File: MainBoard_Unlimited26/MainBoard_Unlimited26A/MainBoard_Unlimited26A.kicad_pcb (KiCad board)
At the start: 2 copper layers, 95 x 60 mm, 39 parts, among them J1 XT, J2 Screw_Terminal_01x02, J3 BAT, J4 EN, J5 UART, J6 UART, J7 VL5, P1 MP1584, P2 SERVO, Q1 IRFZ44N, U11 ACS712xLCTR-05B, U7 ESP32-DEVKIT-V1, U8 MPU6050/BNO085 I2C, U9 AMS1117-3.3

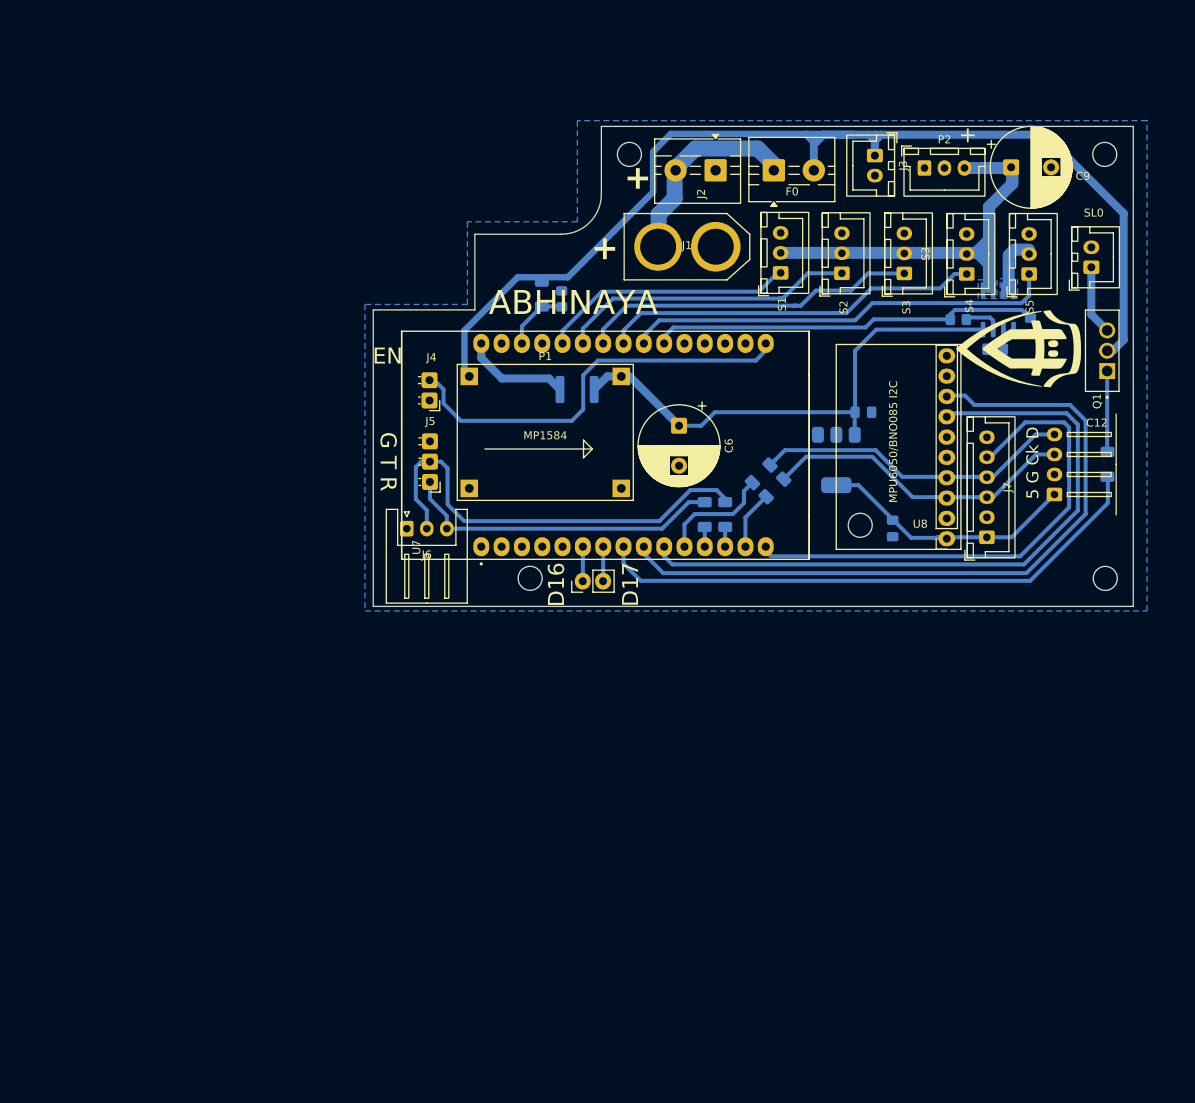
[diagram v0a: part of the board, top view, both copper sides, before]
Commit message: REV ALL
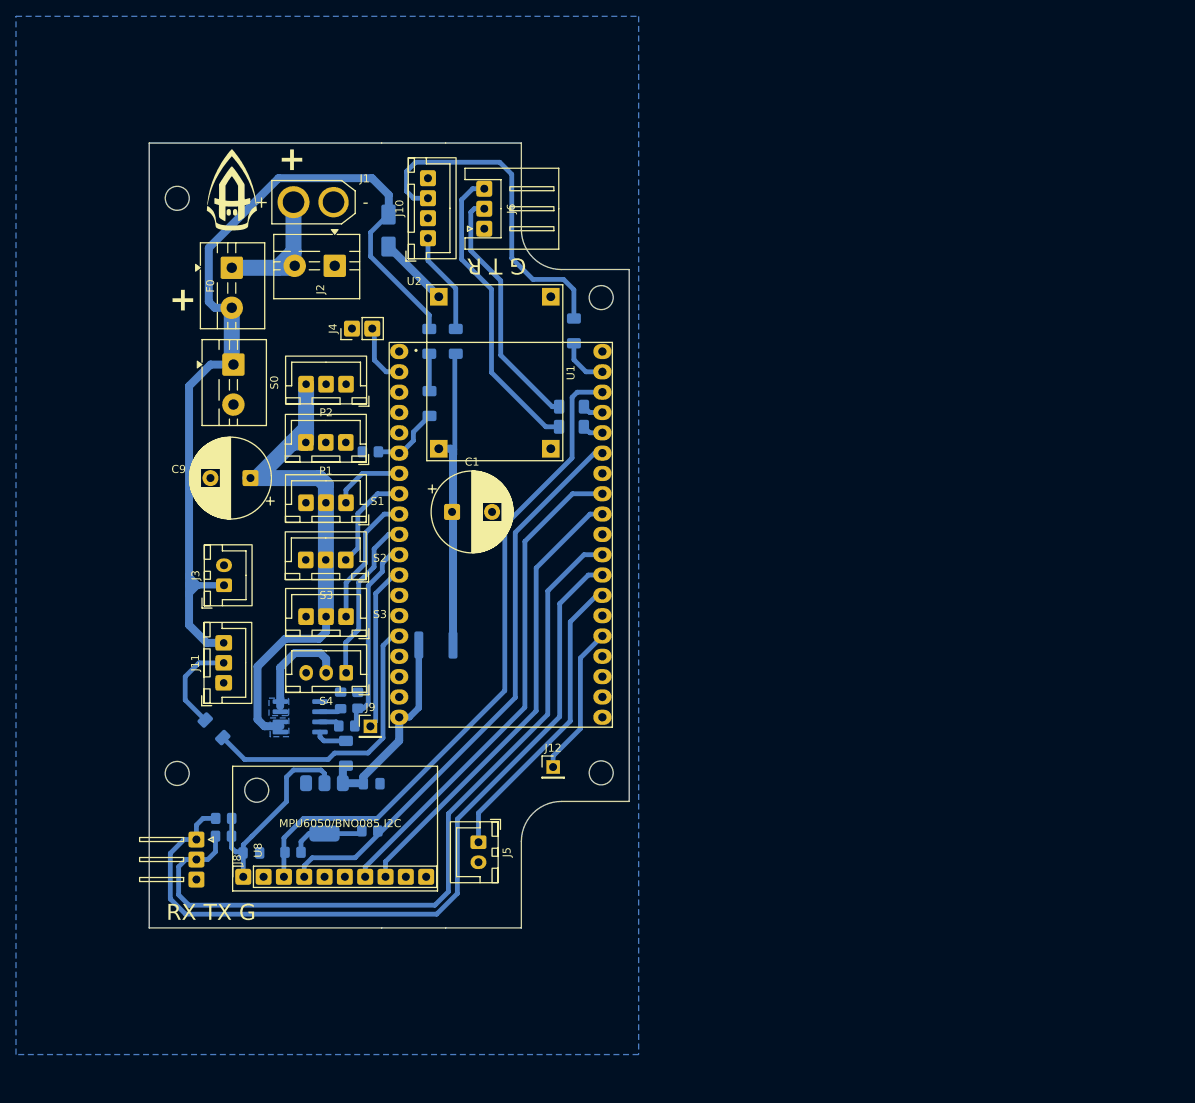
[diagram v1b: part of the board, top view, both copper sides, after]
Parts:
- removed C12: AB conn, Connector_JST:JST_XH_S4B-XH-A-1_1x04_P2.50mm_Horizontal
- removed C6: 1000uF, Capacitor_THT:CP_Radial_D10.0mm_P5.00mm
- removed D16: pin, Connector_PinHeader_2.54mm:PinHeader_1x02_P2.54mm_Vertical
- removed F6: Polyfuse, Fuse:Fuse_1812_4532Metric
- removed J7: VL5, Connector_JST:JST_XH_B6B-XH-A_1x06_P2.50mm_Vertical
- removed Q1: IRFZ44N, IRFZ44N:TO254P1016X419X2286-3
- removed S5: SERVO, Connector_JST:JST_XH_B3B-XH-A_1x03_P2.50mm_Vertical
- removed SL0: SELONOID, Connector_JST:JST_XH_B2B-XH-A_1x02_P2.50mm_Vertical
- removed U7: ESP32-DEVKIT-V1, ESP32-Devkit-V1:MODULE_ESP32_DEVKIT_V1
- added C1: 1000uF, Capacitor_THT:CP_Radial_D10.0mm_P5.00mm, F.Cu at (98.4, 108.2)
- added D2: D, Diode_SMD:D_SMA, B.Cu at (90.5, 73.0)
- added F1: Polyfuse, Fuse:Fuse_1812_4532Metric, B.Cu at (96.4, 124.8)
- added J10: relay, Connector_JST:JST_XH_B4B-XH-A_1x04_P2.50mm_Vertical, F.Cu at (95.4, 73.9)
- added J11: led, Connector_JST:JST_XH_B3B-XH-A_1x03_P2.50mm_Vertical, F.Cu at (69.9, 129.5)
- added J12: Conn_01x01_Socket, Connector_PinHeader_2.54mm:PinHeader_1x01_P2.54mm_Vertical, F.Cu at (111.0, 140.0)
- added J8: UART, Connector_JST:JST_XH_S3B-XH-A-1_1x03_P2.50mm_Horizontal, F.Cu at (66.5, 149.1)
- added J9: Conn_01x01_Socket, Connector_PinHeader_2.54mm:PinHeader_1x01_P2.54mm_Vertical, F.Cu at (88.2, 134.9)
- added R10: 4k7, Resistor_SMD:R_0805_2012Metric_Pad1.20x1.40mm_HandSolder, B.Cu at (88.1, 148.0)
- added R11: 4k7, Resistor_SMD:R_0805_2012Metric_Pad1.20x1.40mm_HandSolder, B.Cu at (78.5, 150.7)
- added R12: 0, Resistor_SMD:R_1206_3216Metric_Pad1.30x1.75mm_HandSolder, B.Cu at (98.9, 86.8)
- added R13: 0, Resistor_SMD:R_1206_3216Metric_Pad1.30x1.75mm_HandSolder, B.Cu at (68.7, 135.3)
- added R14: 10k, Resistor_SMD:R_0805_2012Metric_Pad1.20x1.40mm_HandSolder, B.Cu at (69.9, 146.5)
- added R15: 10k, Resistor_SMD:R_0805_2012Metric_Pad1.20x1.40mm_HandSolder, B.Cu at (69.8, 148.7)
- added S0: Screw_Terminal_01x02, TerminalBlock:TerminalBlock_MaiXu_MX126-5.0-02P_1x02_P5.00mm, F.Cu at (71.1, 89.7)
- added U1: MP1584_3A_Mini, mp1548:MP1584_Module, F.Cu at (103.8, 90.8)
- added U2: ESP32-DEVKITC-32UE, ESP32-Devkit-V1:ESPRESSIF_ESP32-DEVKITC-32UE, F.Cu at (104.5, 111.0)
- J1: footprint Connector_AMASS:AMASS_XT60-M_1x02_P7.20mm_Vertical -> Connector_AMASS:AMASS_XT30U-F_1x02_P5.0mm_Vertical
- J4: footprint Connector_PinHeader_2.54mm:PinHeader_1x02_P2.54mm_Horizontal -> Connector_PinHeader_2.54mm:PinHeader_1x02_P2.54mm_Vertical
- J5: value UART -> Laser; footprint Connector_PinHeader_2.54mm:PinHeader_1x03_P2.54mm_Horizontal -> Connector_JST:JST_XH_B2B-XH-A_1x02_P2.50mm_Vertical
- P1: value MP1584 -> SERVO; footprint mp1548:MP1584_Module -> Connector_JST:JST_XH_B3B-XH-A_1x03_P2.50mm_Vertical
- R3: value 470 -> 0
- R6: value 2K -> 1k
- R7: value 1K -> 2k
- moved C9 102.7 mm to (73.2, 103.9), turned to 180 degrees
- moved U11 101.0 mm to (79.4, 133.8), turned to 0 degrees
- moved G*** 100.3 mm to (70.9, 67.9), turned to 0 degrees
- moved U8 97.6 mm to (72.3, 153.8), turned to 90 degrees
- moved J3 97.5 mm to (69.9, 117.3), turned to 90 degrees
- moved R7 96.2 mm to (86.6, 131.7), turned to -90 degrees
- moved C11 92.8 mm to (84.5, 131.7), turned to 90 degrees
- moved S4 92.2 mm to (85.2, 128.3), turned to 180 degrees
- moved R6 91.8 mm to (85.3, 134.9), turned to 0 degrees
- moved C8 89.8 mm to (73.3, 150.8), turned to 0 degrees
- moved S3 81.9 mm to (85.2, 121.2), turned to 180 degrees
- moved U9 77.4 mm to (82.5, 145.2)
- moved P2 77.2 mm to (85.2, 92.2), turned to 180 degrees
- moved C7 77.0 mm to (88.4, 142.1)
- moved S2 71.6 mm to (85.1, 114.2), turned to 180 degrees
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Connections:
- net D13 renamed D35
- J5 pad 1: RX -> D4
- J5 pad 2: TX -> GND
- P1 pad 1: +12V -> GND
- P1 pad 2: GND -> unconnected-(P1-Pin_2-Pad2)
- P1 pad 3: +5V -> +6V
- R1 pad 1: +12V -> Net-(R1-Pad1)
- R3 pad 1: D5 -> TX
- R4 pad 1: Net-(U7-RX0) -> RX
- R4 pad 2: RX -> Net-(U2-RX)
- R5 pad 1: Net-(U7-TX0) -> Net-(U11-VCC)
- R5 pad 2: TX -> +5V
- R6 pad 2: D32 -> D27
- R7 pad 2: D32 -> D27
- R8 pad 1: SDA -> Net-(U2-23)
- R8 pad 2: Net-(U7-D21) -> 23
- R9 pad 1: Net-(U7-D22) -> Net-(R1-Pad1)
- R9 pad 2: SCL -> +12V
- S1 pad 1: D14 -> D32
- S2 pad 1: D27 -> D33
- S3 pad 1: D26 -> D25
- S4 pad 1: D25 -> D26
- S4 pad 2: +6V -> +6VO
- U11 pad 8: +5V -> Net-(U11-VCC)
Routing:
- net D16R: track 0.00 -> 100.3 mm
- net D17T: track 0.00 -> 97.2 mm
- net D5: track 71.1 -> 0.00 mm
- net D23: track 63.6 -> 0.00 mm
- net SCL: track 39.4 -> 84.3 mm
- net EN: track 52.2 -> 8.49 mm
- net 23: track 0.00 -> 42.6 mm
- net D33: track 53.9 -> 13.1 mm
- net +5Vo: track 0.00 -> 39.4 mm
- net D32: track 49.0 -> 9.59 mm
- net +5V: track 64.2 -> 25.9 mm
- net D4: track 0.00 -> 37.7 mm
- net Net-(U2-13): track 0.00 -> 36.8 mm
- net D18: track 90.5 -> 57.5 mm
- net SDA: track 40.0 -> 72.1 mm
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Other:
- board size 95 x 60 mm -> 60 x 98.1 mm
- board text added: "RX TX G"
- board text removed: "5 G Ck D"
- board text removed: "ABHINAYA"
- board text removed: "D17"
